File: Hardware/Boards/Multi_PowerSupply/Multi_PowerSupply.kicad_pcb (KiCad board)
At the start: 2 copper layers, 75.2 x 76.2 mm, 35 parts, among them J1 Input_1, J10 Output, J11 Conn_01x02_Male, J12 Conn_01x02_Male, J13 Conn_01x02_Male, J14 Conn_01x02_Male, J15 Conn_01x02_Male, J2 Input_2, J3 Input_3, J4 Input_4, J5 Conn_01x02_Male, J6 Conn_01x02_Male, J7 Conn_01x02_Male, J8 Conn_01x02_Male, J9 Conn_01x02_Male

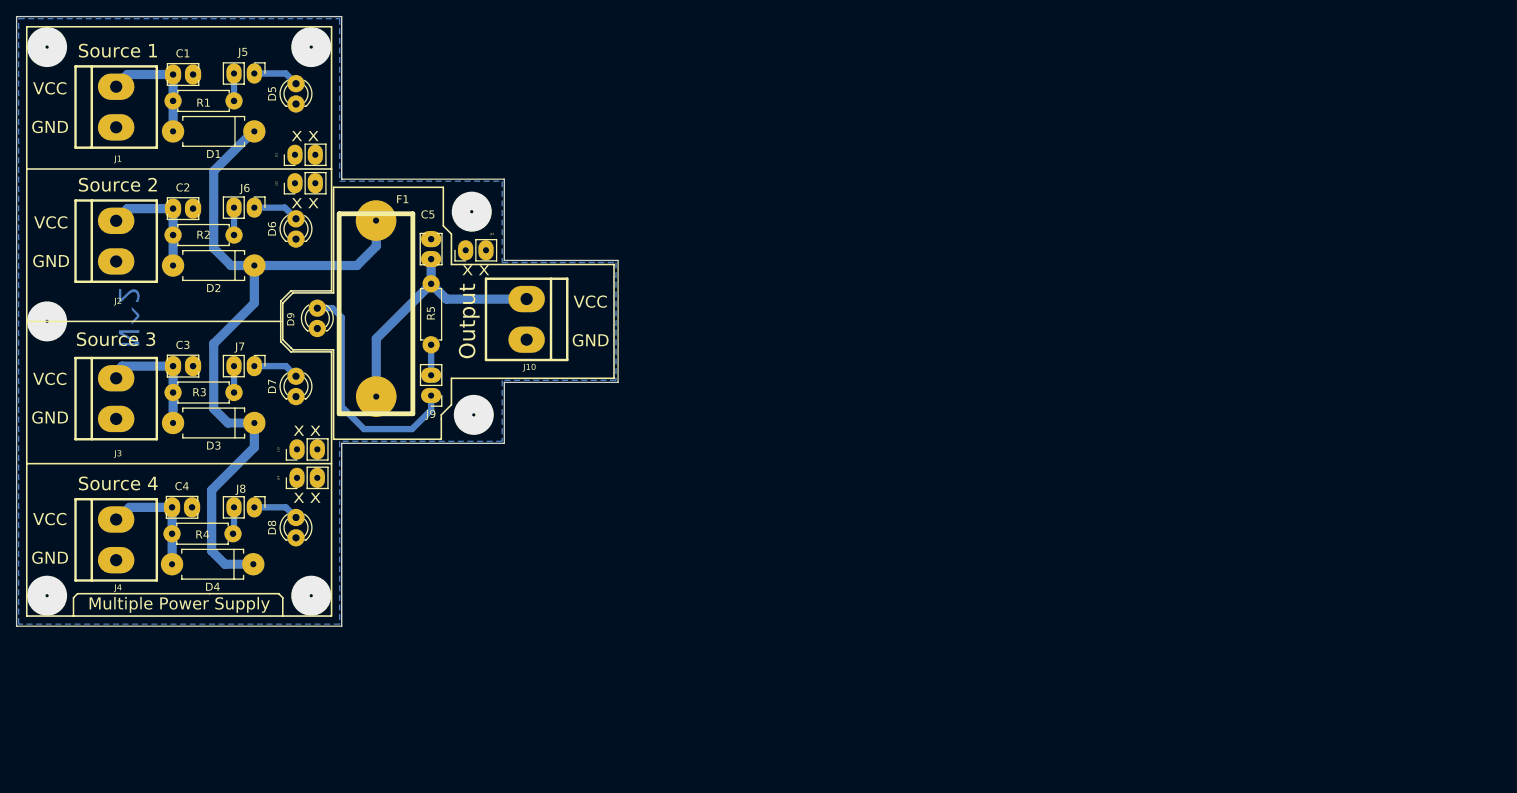
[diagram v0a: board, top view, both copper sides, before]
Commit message: Add boards and report in tex.
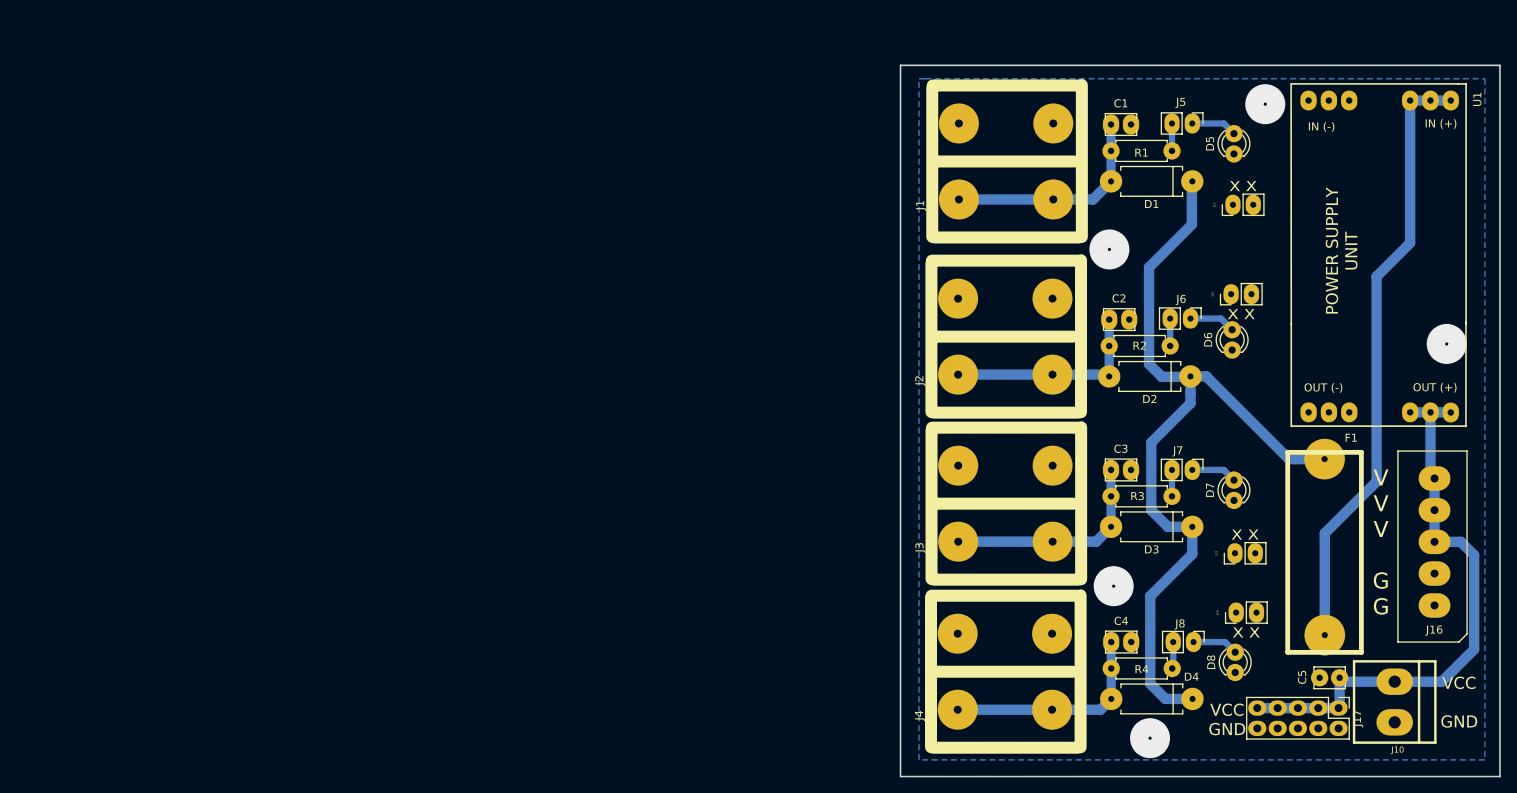
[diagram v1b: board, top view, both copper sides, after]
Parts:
- removed D9: LED, _018:LED_D3.0mm
- removed J15, J9: Conn_01x02_Male, Connector_PinHeader_2.54mm:PinHeader_1x02_P2.54mm_Vertical
- removed R5: R, _018:Res_Small
- added J16: Conn_01x05, _019:Molex_5, F.Cu at (198.8, 95.5)
- added J17: Conn_02x05_Top_Bottom, Connector_PinHeader_2.54mm:PinHeader_2x05_P2.54mm_Vertical, F.Cu at (186.8, 108.3)
- added U1: Buck, _018:Buck_Regulator, F.Cu at (200.9, 32.3)
- J1, J2, J3, J4: footprint _018:bornier2-medium -> _018:Solar_Connector
- moved C5 125.0 mm to (187.0, 104.5), turned to 180 degrees
- moved F1 122.3 mm to (184.6, 88.6)
- moved R4 118.6 mm to (166.0, 103.3)
- moved C4 118.6 mm to (158.4, 100.0)
- moved D4 118.6 mm to (168.6, 107.1)
- moved D8 118.6 mm to (173.9, 103.8)
- moved J14 118.6 mm to (174.0, 96.3)
- moved J8 118.6 mm to (168.7, 100.0)
- moved J10 118.6 mm to (193.9, 107.5)
- moved D7 118.0 mm to (173.8, 82.3)
- moved C3 118.0 mm to (158.4, 78.5)
- moved D3 118.0 mm to (168.6, 85.6)
- moved J13 118.0 mm to (173.9, 88.9)
- moved J7 118.0 mm to (168.6, 78.5)
- moved R3 118.0 mm to (166.0, 81.8)
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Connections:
- C5 pad 1: Net-(C5-Pad1) -> VCC
- F1 pad 1: Net-(C5-Pad1) -> Net-(F1-Pad1)
- J10 pad 2: Net-(C5-Pad1) -> VCC
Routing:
- net Net-(F1-Pad1): track 0.00 -> 76.3 mm
- net VCC: track 0.00 -> 71.6 mm
- net Net-(C5-Pad1): track 32.8 -> 0.00 mm
- net Net-(D9-Pad2): track 29.8 -> 0.00 mm
- net Net-(D1-Pad1): track 92.1 -> 104.7 mm
- net Net-(C4-Pad1): track 14.7 -> 26.9 mm
- net Net-(C1-Pad1): track 14.9 -> 27.1 mm
- net Net-(C3-Pad1): track 15.3 -> 27.0 mm
- net Net-(C2-Pad1): track 14.9 -> 26.1 mm
- net Net-(J9-Pad2): track 3.81 -> 0.00 mm
- net (no net): vias 7 -> 5
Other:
- board size 75.2 x 76.2 mm -> 74.9 x 88.9 mm
- net class Power: trace_width 1.1455 -> 1.295
- board text added: "POWER SUPPLY UNIT"
- board text added: "V V V G G"
- board text removed: "Multiple Power Supply"
- board text removed: "N^2"
- board text removed: "Output"
- board text removed: "Source 1"
- board text removed: "Source 2"
- board text removed: "Source 3"
- board text removed: "Source 4"
